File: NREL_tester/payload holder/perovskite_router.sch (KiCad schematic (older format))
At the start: 3 parts, among them J1 Conn_01x10_Male, J2 Conn_01x10_Male, J3 Conn_01x11_Male

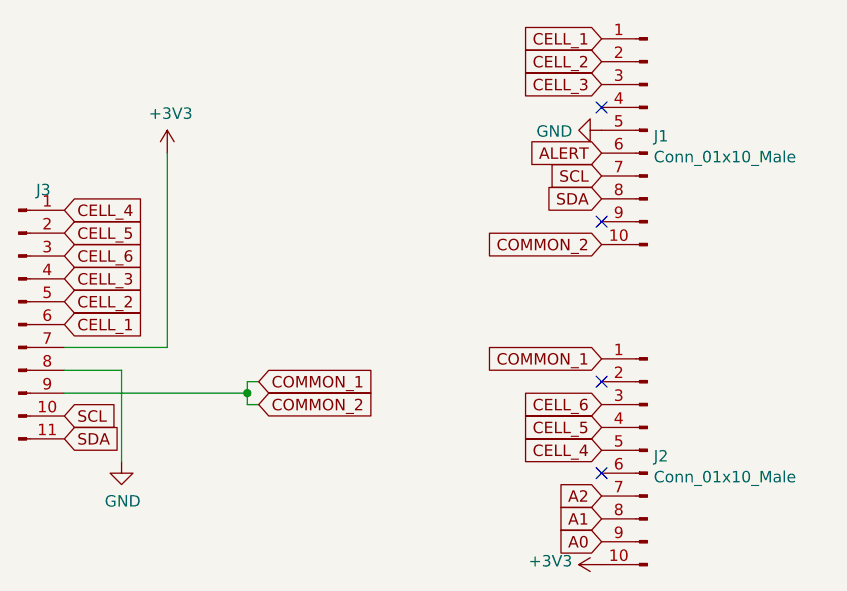
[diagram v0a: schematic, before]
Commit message: Flight computer v2 complete
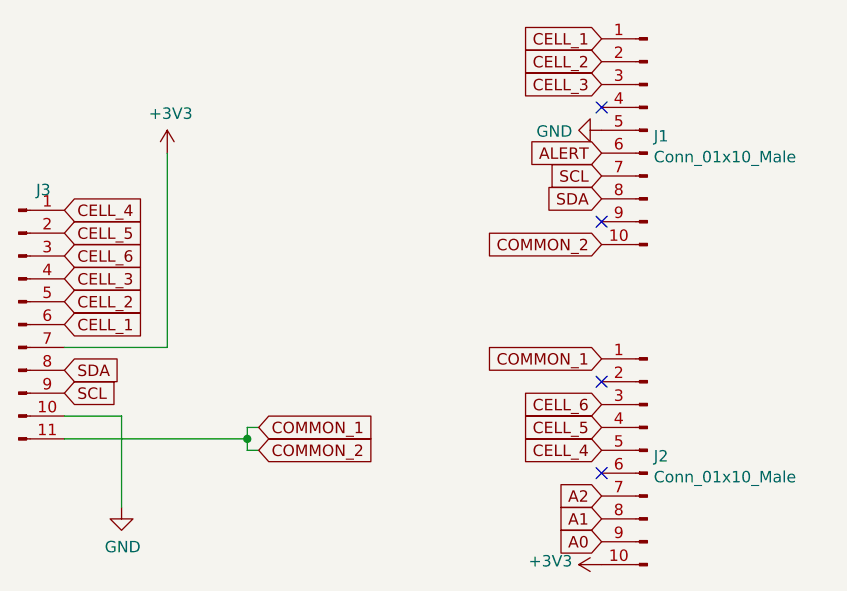
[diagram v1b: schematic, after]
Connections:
- net COMMON_1: now also J3.11 (Pin_11); no longer J3.9 (Pin_9)
- net GND: now also J3.10 (Pin_10); no longer J3.8 (Pin_8)
- net SCL: now also J3.9 (Pin_9); no longer J3.10 (Pin_10)
- net SDA: now also J3.8 (Pin_8); no longer J3.11 (Pin_11)
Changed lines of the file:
@@
 L power:GND #PWR0106
 U 1 1 64AB952A
-P 4850 4800
-F 0 "#PWR0106" H 4850 4550 50  0001 C CNN
-F 1 "GND" H 4855 4627 50  0000 C CNN
-F 2 "" H 4850 4800 50  0001 C CNN
-F 3 "" H 4850 4800 50  0001 C CNN
-	1    4850 4800
+P 4850 5000
+F 0 "#PWR0106" H 4850 4750 50  0001 C CNN
+F 1 "GND" H 4855 4827 50  0000 C CNN
+F 2 "" H 4850 5000 50  0001 C CNN
+F 3 "" H 4850 5000 50  0001 C CNN
+	1    4850 5000
 	1    0    0    -1
 $EndComp
-Text GLabel 4600 4700 2    50   Input ~ 0
+Text GLabel 4600 4400 2    50   Input ~ 0
 SDA
-Text GLabel 4600 4600 2    50   Input ~ 0
+Text GLabel 4600 4500 2    50   Input ~ 0
 SCL
 Text GLabel 4600 4200 2    50   Input ~ 0
@@
 Text GLabel 4600 3700 2    50   Input ~ 0
 CELL_4
-Text GLabel 5450 4450 2    50   Input ~ 0
+Text GLabel 5450 4650 2    50   Input ~ 0
 COMMON_1
-Text GLabel 5450 4550 2    50   Input ~ 0
+Text GLabel 5450 4750 2    50   Input ~ 0
 COMMON_2
 $Comp
@@
 $EndComp
 Wire Wire Line
-	5450 4450 5400 4450
+	5450 4650 5400 4650
 Wire Wire Line
-	5400 4450 5400 4500
+	5400 4650 5400 4700
 Wire Wire Line
-	5400 4550 5450 4550
+	5400 4750 5450 4750
 Wire Wire Line
-	5400 4500 4600 4500
-Connection ~ 5400 4500
+	5400 4700 4600 4700
+Connection ~ 5400 4700
 Wire Wire Line
-	5400 4500 5400 4550
+	5400 4700 5400 4750
 Wire Wire Line
-	4600 4400 4850 4400
+	4600 4600 4850 4600
 Wire Wire Line
-	4850 4400 4850 4800
+	4850 4600 4850 5000
 Wire Wire Line
 	4600 4300 5050 4300
